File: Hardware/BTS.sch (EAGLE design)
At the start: 55 parts, among them IC1 TPA3140D2PWP, IC2 BLK-MD-SPK-B, J1 SPKR_OUT, J2 RN52BoB_R, J3 RN52BoB_L, J6 HC-05, J7 PRT-10474, T3_2 TEENSY_3.1-3.2_DIL

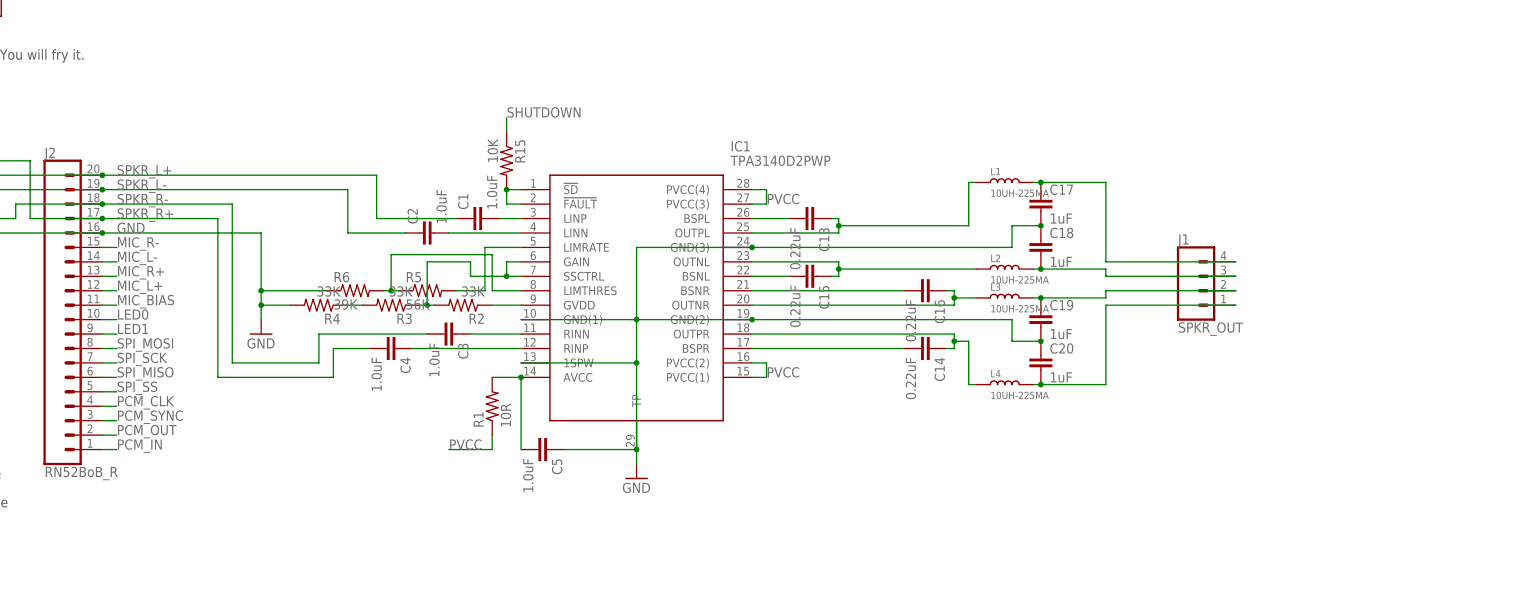
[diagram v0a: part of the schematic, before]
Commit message: Still working on figuring out an error w/ the board
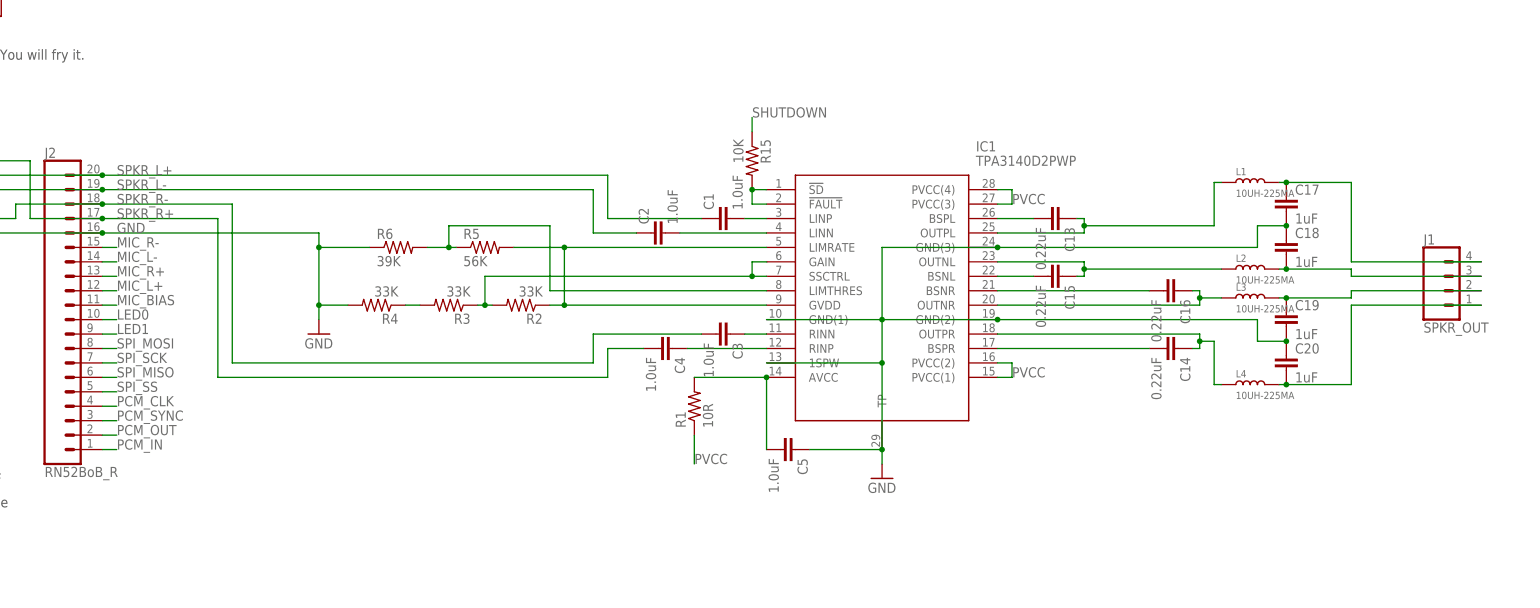
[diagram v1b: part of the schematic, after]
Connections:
- removed net LIMRATE: IC1.LIMRATE, R5.2
- net GVDD: now also IC1.LIMRATE, R5.2
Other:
- moved on the sheet: C1, C13, C14, C15, C16, C17, C18, C19, C2, C20, C3, C4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
